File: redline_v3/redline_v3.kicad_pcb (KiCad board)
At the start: 2 copper layers, 78.8 x 97.5 mm, 69 parts, among them J1 Conn_01x10_Socket, J2 Conn_01x10_Socket

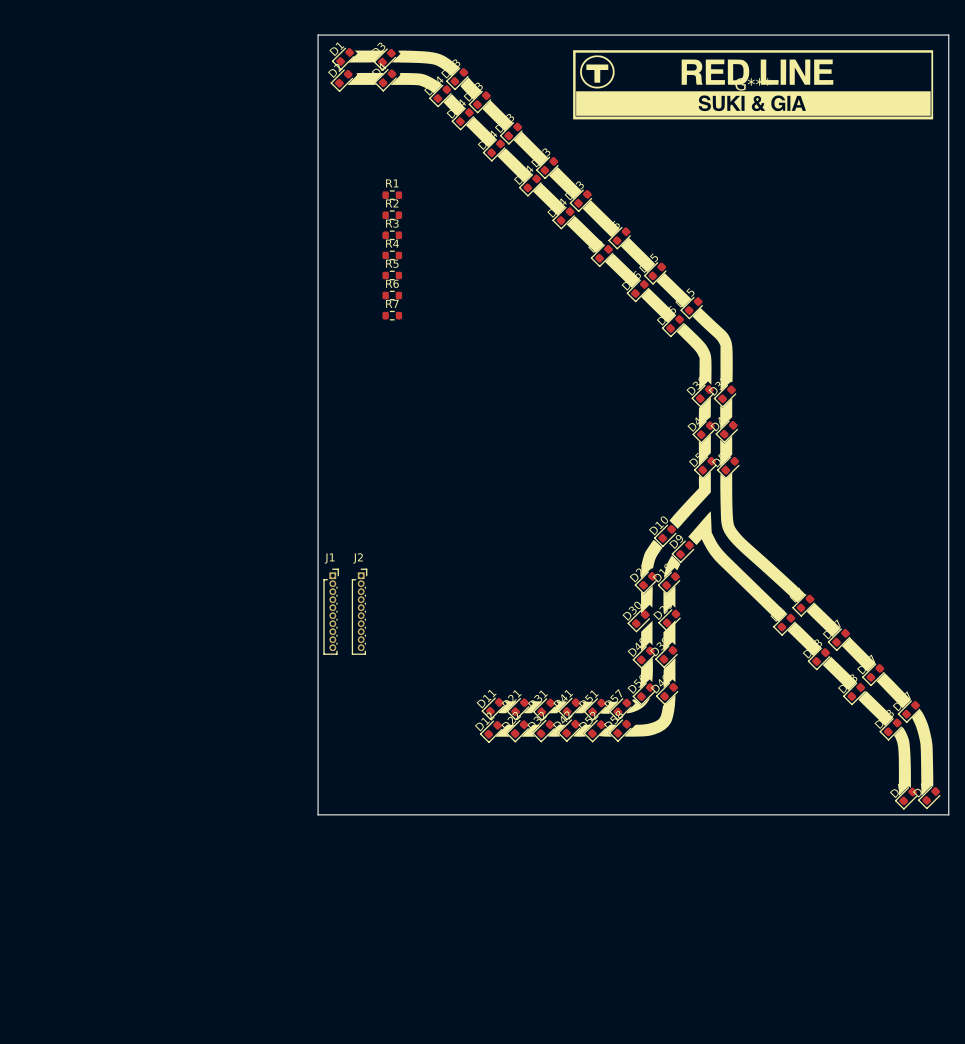
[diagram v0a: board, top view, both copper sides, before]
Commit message: traces all done
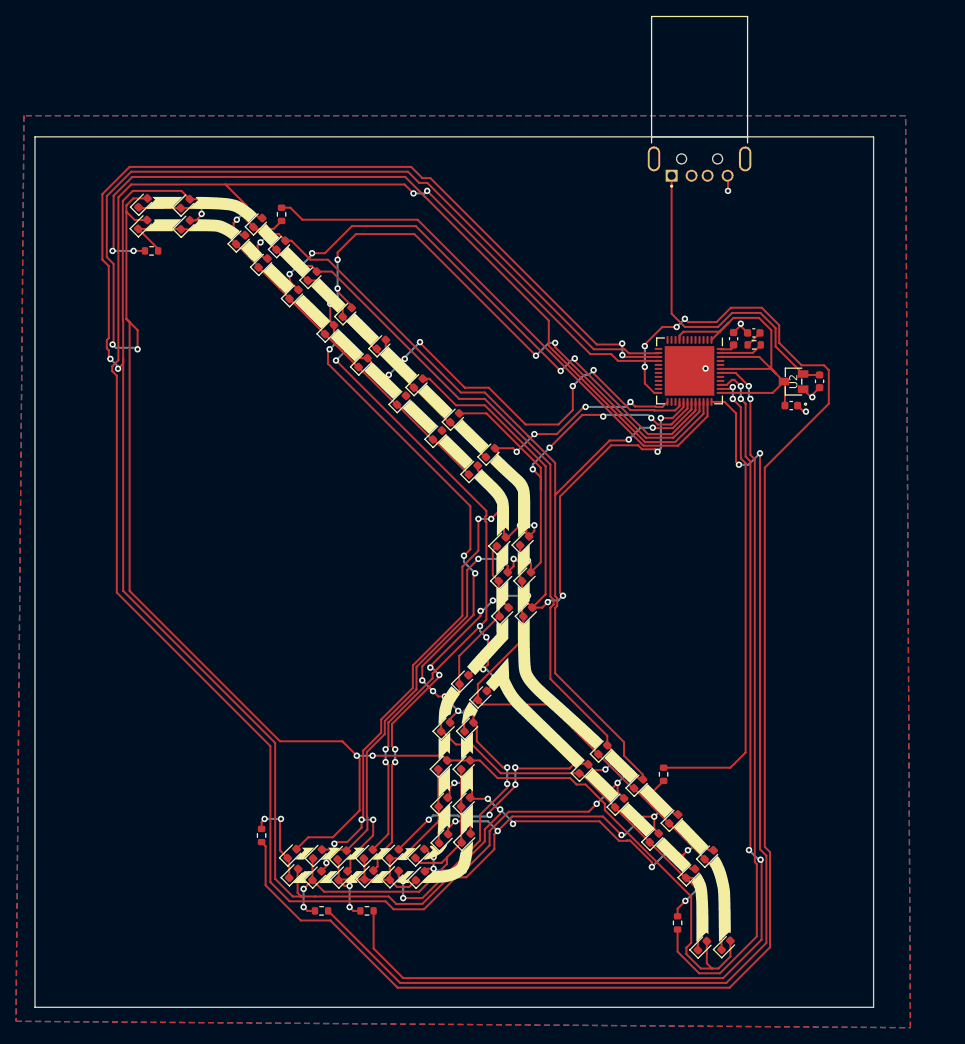
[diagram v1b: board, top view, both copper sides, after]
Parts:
- removed the G*** at (222.9, 45.7)
- removed J1, J2: Conn_01x10_Socket, Connector_PinSocket_1.00mm:PinSocket_1x10_P1.00mm_Vertical
- added C1: 10nF, Capacitor_SMD:C_0603_1608Metric, F.Cu at (220.5, 77.5)
- added C2: 3.3nF, Capacitor_SMD:C_0603_1608Metric, F.Cu at (223.0, 76.8)
- added C3: C_1uF, footprints:C_0603_1608Metric, F.Cu at (231.2, 82.8)
- added C4: C_1uF, footprints:C_0603_1608Metric, F.Cu at (227.7, 85.8)
- added J4: 48037-0001, custom_library:MOLEX_USB_conn, F.Cu at (216.2, 55.0)
- added R8: R_US, Resistor_SMD:R_0603_1608Metric, F.Cu at (223.1, 78.2)
- added U1: ESP32, Package_DFN_QFN:QFN-48-1EP_8x8mm_P0.5mm_EP6.2x6.2mm, F.Cu at (215.0, 81.5)
- added U2: MCP1702T-3302E_MB, custom_library:MCP1702T, F.Cu at (228.0, 82.8)
- moved D23 110.0 mm to (219.5, 153.3)
- moved D33 104.5 mm to (216.6, 153.3)
- moved D1 99.8 mm to (165.3, 141.8)
- moved D2 99.5 mm to (165.5, 144.3)
- moved D24 97.1 mm to (217.4, 142.0)
- moved D34 93.8 mm to (215.1, 144.3)
- moved R5 88.4 mm to (213.5, 150.5), turned to 90 degrees
- moved R1 81.7 mm to (161.5, 139.6), turned to 90 degrees
- moved D17 80.1 mm to (167.8, 69.6)
- moved D44 78.2 mm to (184.2, 135.4)
- moved R6 77.0 mm to (174.7, 149.0), turned to 180 degrees
- moved D43 76.1 mm to (184.1, 130.8)
- moved R7 74.9 mm to (169.0, 149.0), turned to 180 degrees
- moved D7 74.7 mm to (165.5, 71.9)
- moved D54 74.3 mm to (187.0, 135.4)
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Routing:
- net /1: track 0.00 -> 298.4 mm, vias 0 -> 15
- net /0: track 0.00 -> 284.1 mm, vias 0 -> 4
- net /2: track 0.00 -> 255.7 mm, vias 0 -> 11
- net /A: track 0.00 -> 188.6 mm, vias 0 -> 4
- net /4: track 0.00 -> 186.6 mm, vias 0 -> 11
- net /5: track 0.00 -> 175.5 mm, vias 0 -> 18
- net /3: track 0.00 -> 157.8 mm, vias 0 -> 11
- net /6: track 0.00 -> 150.6 mm, vias 0 -> 13
- net /G: track 0.00 -> 135.6 mm, vias 0 -> 2
- net /F: track 0.00 -> 130.4 mm, vias 0 -> 4
- net /7: track 0.00 -> 128.4 mm, vias 0 -> 12
- net /9: track 0.00 -> 120.0 mm, vias 0 -> 12
- net /8: track 0.00 -> 111.2 mm, vias 0 -> 8
- net /B: track 0.00 -> 104.3 mm, vias 0 -> 2
- net /E: track 0.00 -> 89.1 mm, vias 0 -> 2
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- added copper zone on B.Cu, net (none)
- added copper zone on F.Cu, net (none)
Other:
- board size 78.8 x 97.5 mm -> 104.8 x 108.8 mm
